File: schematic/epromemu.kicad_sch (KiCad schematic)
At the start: 19 parts, among them J3 EPROM Connector, U1 Teensy4.1, U2 74HC245, U3 74HC245, U4 74HC245, U5 74HC245, U6 74HC32

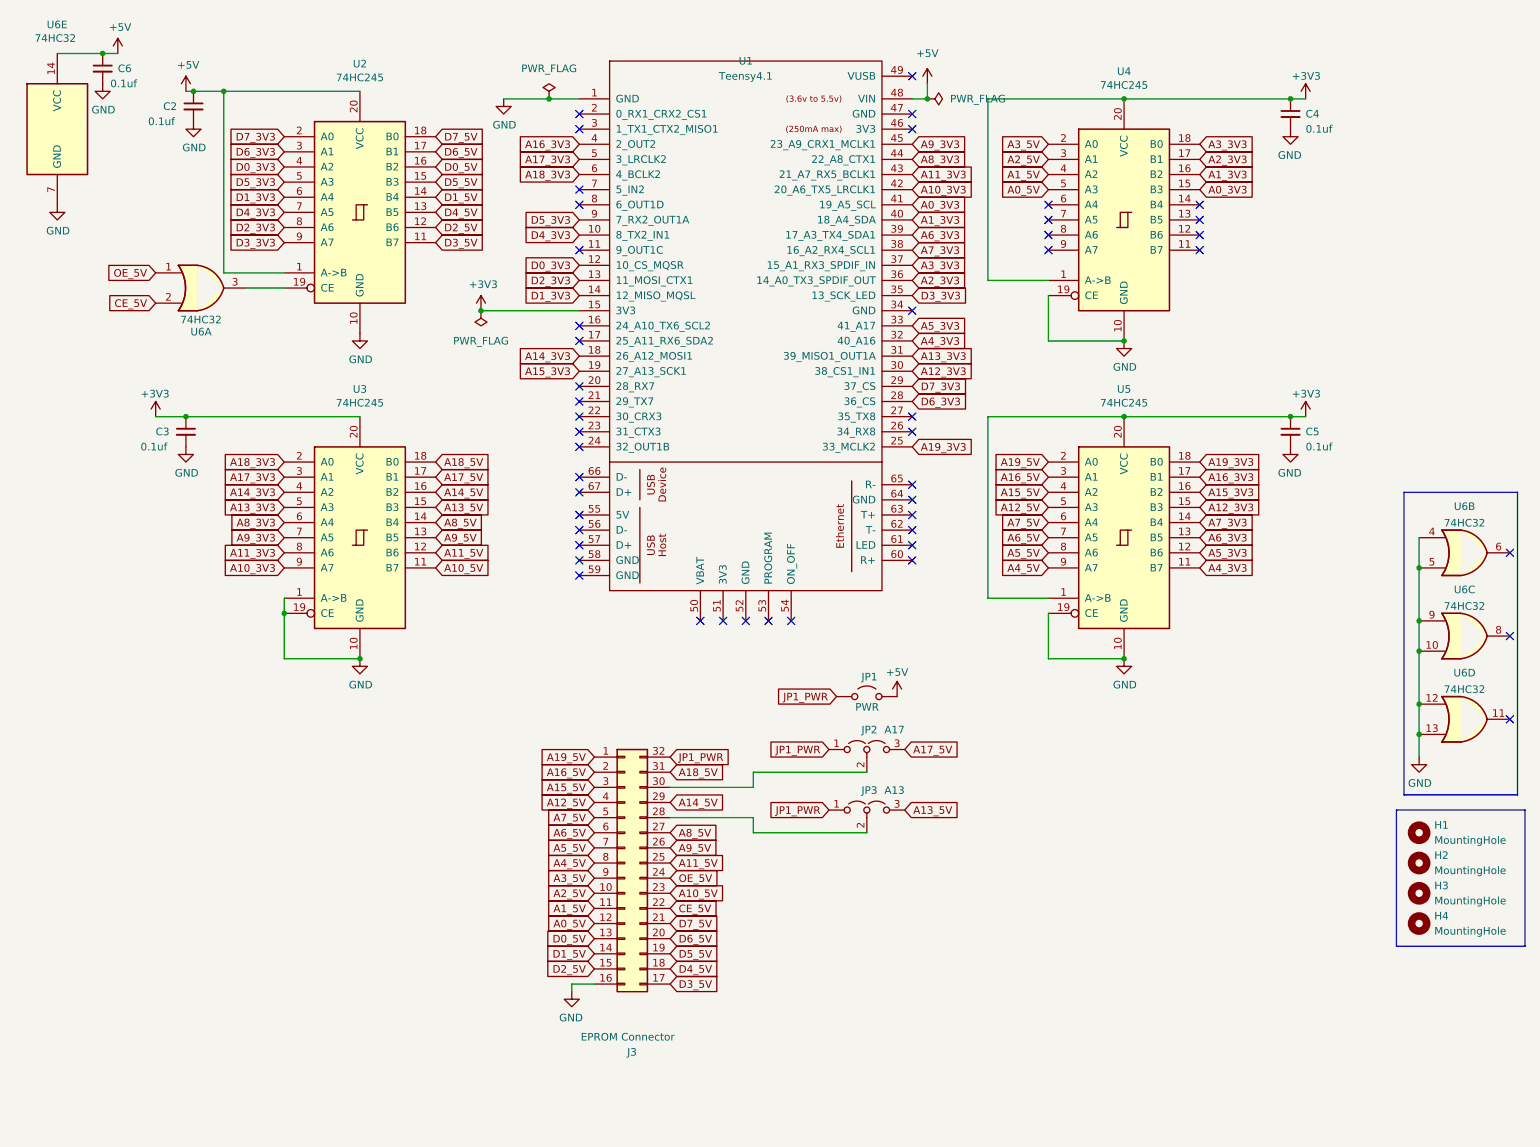
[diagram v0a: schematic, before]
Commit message: REV D
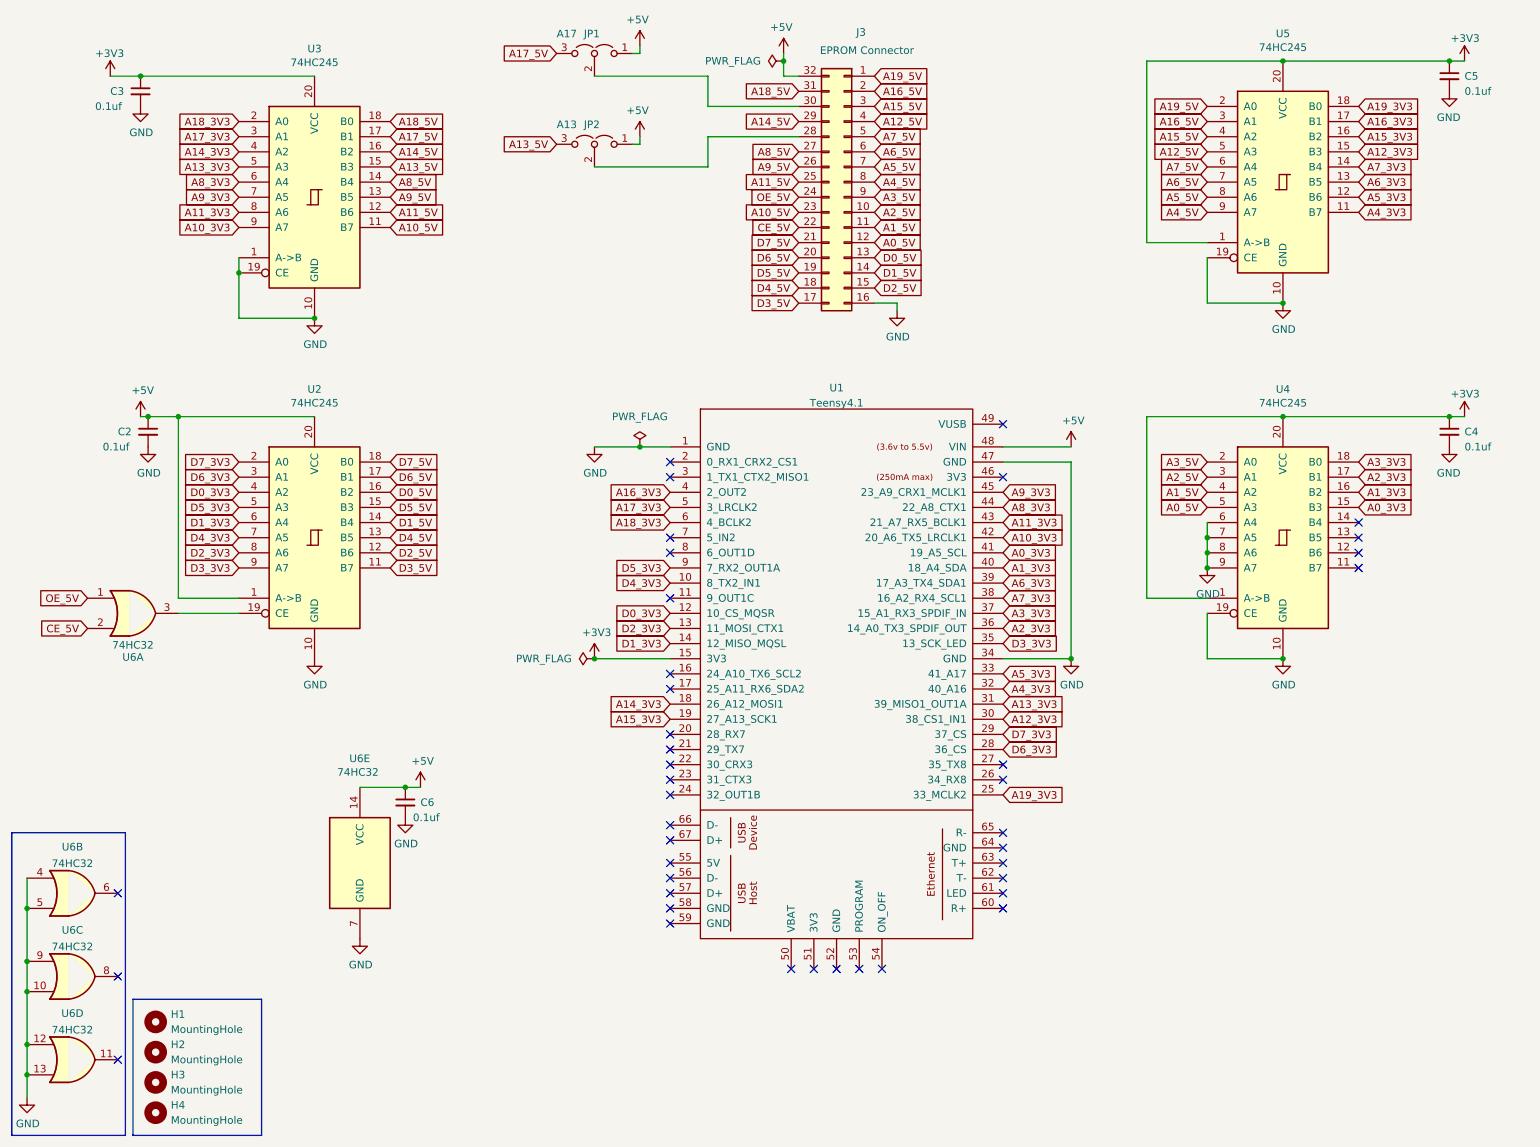
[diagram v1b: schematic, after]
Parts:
- removed JP1: PWR, Connector_PinHeader_2.54mm:PinHeader_1x02_P2.54mm_Vertical, symbol Jumper:Jumper_2_Open
- JP1: renamed from JP2; footprint Connector_PinHeader_2.54mm:PinHeader_1x03_P2.54mm_Vertical -> MyFootprints:Jumper_1x03_P2.54mm_Vertical
- JP2: renamed from JP3; footprint Connector_PinHeader_2.54mm:PinHeader_1x03_P2.54mm_Vertical -> MyFootprints:Jumper_1x03_P2.54mm_Vertical
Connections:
- net JP1_PWR is gone; now on net +5V: J3.32 (Pin_32), JP1.1 (A), JP2.1 (A)
- net GND: now also U1.34 (GND), U1.47 (GND), U4.6 (A4), U4.7 (A5), U4.8 (A6), U4.9 (A7)
- no-connect marks 47 -> 41
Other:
- moved on the sheet: C2, C3, C4, C5, C6, H1, H2, H3, H4, J3, JP1, JP2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
